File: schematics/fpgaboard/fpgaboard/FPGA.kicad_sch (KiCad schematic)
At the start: 15 parts, among them J1 SODIMM-200, U1 LFE5UM-85F-8BG381I, U13 W25Q32JVSS

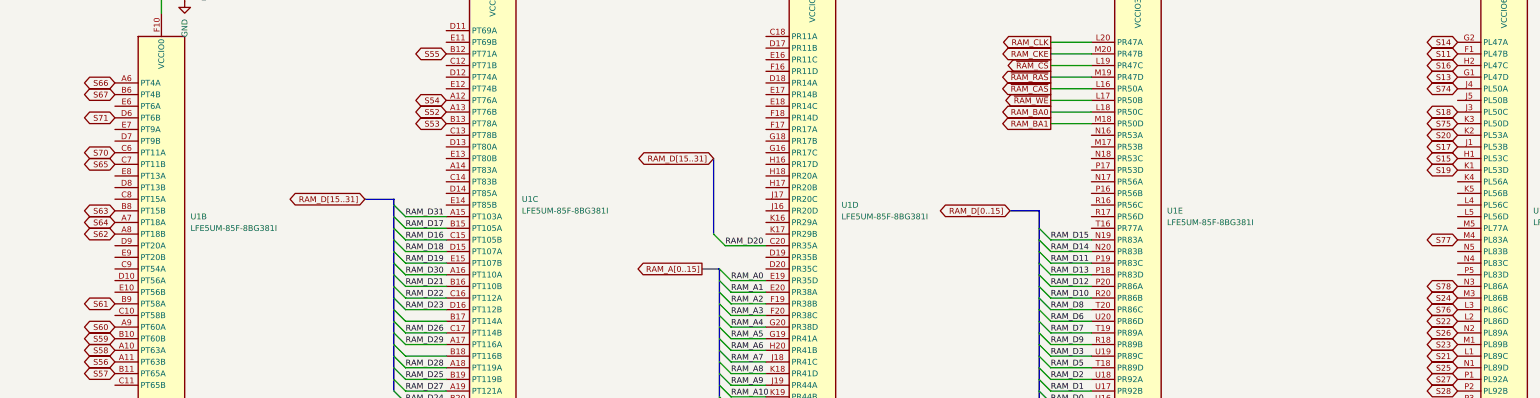
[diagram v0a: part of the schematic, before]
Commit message: Some work on FPGA board.
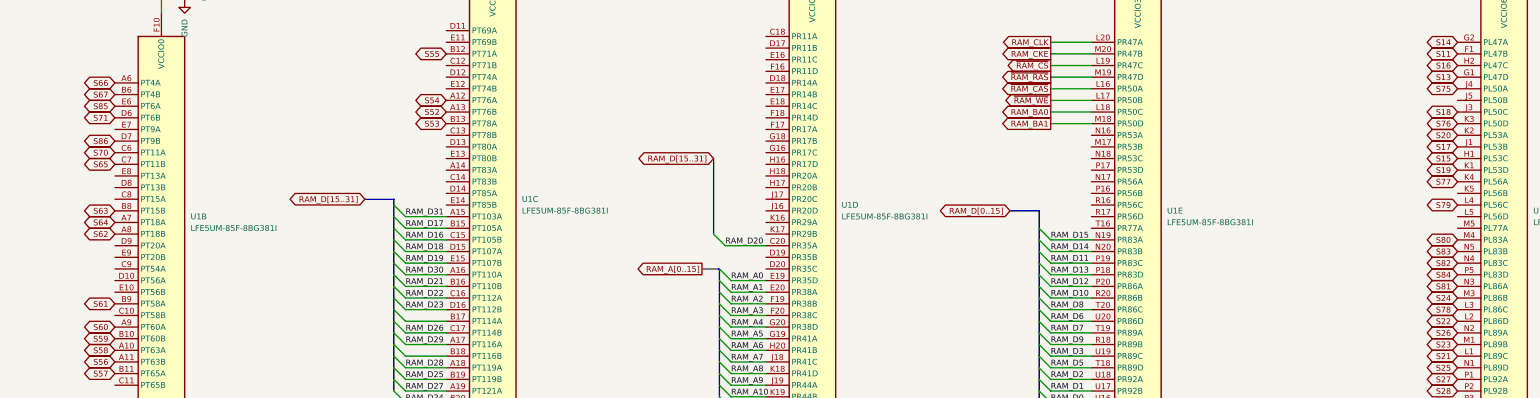
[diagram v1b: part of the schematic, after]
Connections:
- net S74: no longer U1.J4 (PL50A)
- net S75: now also U1.J4 (PL50A); no longer U1.K3 (PL50D)
- net S76: now also U1.K3 (PL50D); no longer U1.L3 (PL86C)
- net S77: now also U1.K4 (PL56A); no longer U1.M4 (PL83A)
- net S78: now also U1.L3 (PL86C); no longer U1.N3 (PL86A)
- net S79: now also U1.L4 (PL56C)
- net S80: now also U1.M4 (PL83A)
- net S81: now also U1.N3 (PL86A)
- net S82: now also U1.N4 (PL83C)
- net S83: now also U1.N5 (PL83B)
- net S84: now also U1.P5 (PL83D)
- net S85: now also U1.E6 (PT6A)
- net S86: now also U1.D7 (PT9B)
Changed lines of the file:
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@@
 		)
 	)
+	(global_label "S80"
+		(shape bidirectional)
+		(at 341.63 107.95 180)
+		(fields_autoplaced yes)
+		(effects
+			(font
+				(size 1.27 1.27)
+			)
+			(justify right)
+		)
+		(property "Intersheetrefs" "${INTERSHEET_REFS}"
+			(at 333.905 107.95 0)
+			(effects
+				(font
+					(size 1.27 1.27)
+				)
+				(justify right)
+				(hide yes)
+			)
+		)
+	)
 	(global_label "S29"
 		(shape bidirectional)
@@
 		)
 	)
-	(global_label "S74"
+	(global_label "S75"
 		(shape bidirectional)
 		(at 341.63 74.93 180)
@@
 		)
 	)
+	(global_label "S86"
+		(shape bidirectional)
+		(at 48.26 86.36 180)
+		(fields_autoplaced yes)
+		(effects
+			(font
+				(size 1.27 1.27)
+			)
+			(justify right)
+		)
+		(property "Intersheetrefs" "${INTERSHEET_REFS}"
+			(at 40.535 86.36 0)
+			(effects
+				(font
+					(size 1.27 1.27)
+				)
+				(justify right)
+				(hide yes)
+			)
+		)
+	)
 	(global_label "S63"
 		(shape bidirectional)
@@
 		)
 	)
+	(global_label "S81"
+		(shape bidirectional)
+		(at 341.63 118.11 180)
+		(fields_autoplaced yes)
+		(effects
+			(font
+				(size 1.27 1.27)
+			)
+			(justify right)
+		)
+		(property "Intersheetrefs" "${INTERSHEET_REFS}"
+			(at 333.905 118.11 0)
+			(effects
+				(font
+					(size 1.27 1.27)
+				)
+				(justify right)
+				(hide yes)
+			)
+		)
+	)
 	(global_label "S17"
 		(shape bidirectional)
@@
 		)
 	)
+	(global_label "S84"
+		(shape bidirectional)
+		(at 341.63 115.57 180)
+		(fields_autoplaced yes)
+		(effects
+			(font
+				(size 1.27 1.27)
+			)
+			(justify right)
+		)
+		(property "Intersheetrefs" "${INTERSHEET_REFS}"
+			(at 333.905 115.57 0)
+			(effects
+				(font
+					(size 1.27 1.27)
+				)
+				(justify right)
+				(hide yes)
+			)
+		)
+	)
 	(global_label "S26"
 		(shape bidirectional)
@@
 		)
 	)
+	(global_label "S85"
+		(shape bidirectional)
+		(at 48.26 78.74 180)
+		(fields_autoplaced yes)
+		(effects
+			(font
+				(size 1.27 1.27)
+			)
+			(justify right)
+		)
+		(property "Intersheetrefs" "${INTERSHEET_REFS}"
+			(at 40.535 78.74 0)
+			(effects
+				(font
+					(size 1.27 1.27)
+				)
+				(justify right)
+				(hide yes)
+			)
+		)
+	)
 	(global_label "S36"
 		(shape bidirectional)
@@
 		)
 	)
+	(global_label "S83"
+		(shape bidirectional)
+		(at 341.63 110.49 180)
+		(fields_autoplaced yes)
+		(effects
+			(font
+				(size 1.27 1.27)
+			)
+			(justify right)
+		)
+		(property "Intersheetrefs" "${INTERSHEET_REFS}"
+			(at 333.905 110.49 0)
+			(effects
+				(font
+					(size 1.27 1.27)
+				)
+				(justify right)
+				(hide yes)
+			)
+		)
+	)
 	(global_label "1v1"
 		(shape input)
@@
 		)
 	)
-	(global_label "S76"
+	(global_label "S77"
 		(shape bidirectional)
-		(at 341.63 123.19 180)
+		(at 341.63 95.25 180)
 		(fields_autoplaced yes)
 		(effects
@@
 		)
 		(property "Intersheetrefs" "${INTERSHEET_REFS}"
-			(at 333.905 123.19 0)
+			(at 333.905 95.25 0)
 			(effects
 				(font
@@
 		)
 	)
+	(global_label "S82"
+		(shape bidirectional)
+		(at 341.63 113.03 180)
+		(fields_autoplaced yes)
+		(effects
+			(font
+				(size 1.27 1.27)
+			)
+			(justify right)
+		)
+		(property "Intersheetrefs" "${INTERSHEET_REFS}"
+			(at 333.905 113.03 0)
+			(effects
+				(font
+					(size 1.27 1.27)
+				)
+				(justify right)
+				(hide yes)
+			)
+		)
+	)
 	(global_label "S83"
 		(shape bidirectional)
@@
 		)
 	)
-	(global_label "S78"
+	(global_label "S79"
 		(shape bidirectional)
-		(at 341.63 118.11 180)
+		(at 341.63 100.33 180)
 		(fields_autoplaced yes)
 		(effects
@@
 		)
 		(property "Intersheetrefs" "${INTERSHEET_REFS}"
-			(at 333.905 118.11 0)
+			(at 333.905 100.33 0)
 			(effects
 				(font
@@
 		)
 	)
-	(global_label "S75"
+	(global_label "S76"
 		(shape bidirectional)
 		(at 341.63 82.55 180)
@@
 		)
 	)
-	(global_label "S77"
+	(global_label "S78"
 		(shape bidirectional)
-		(at 341.63 107.95 180)
+		(at 341.63 123.19 180)
 		(fields_autoplaced yes)
 		(effects
@@
 		)
 		(property "Intersheetrefs" "${INTERSHEET_REFS}"
-			(at 333.905 107.95 0)
+			(at 333.905 123.19 0)
 			(effects
 				(font
